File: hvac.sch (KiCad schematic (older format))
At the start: 18 parts, among them IC1 ATMEGA328P-A, J1 PROGRAMMING HEADER, J2 SERIAL PORT, U1 MIC5225

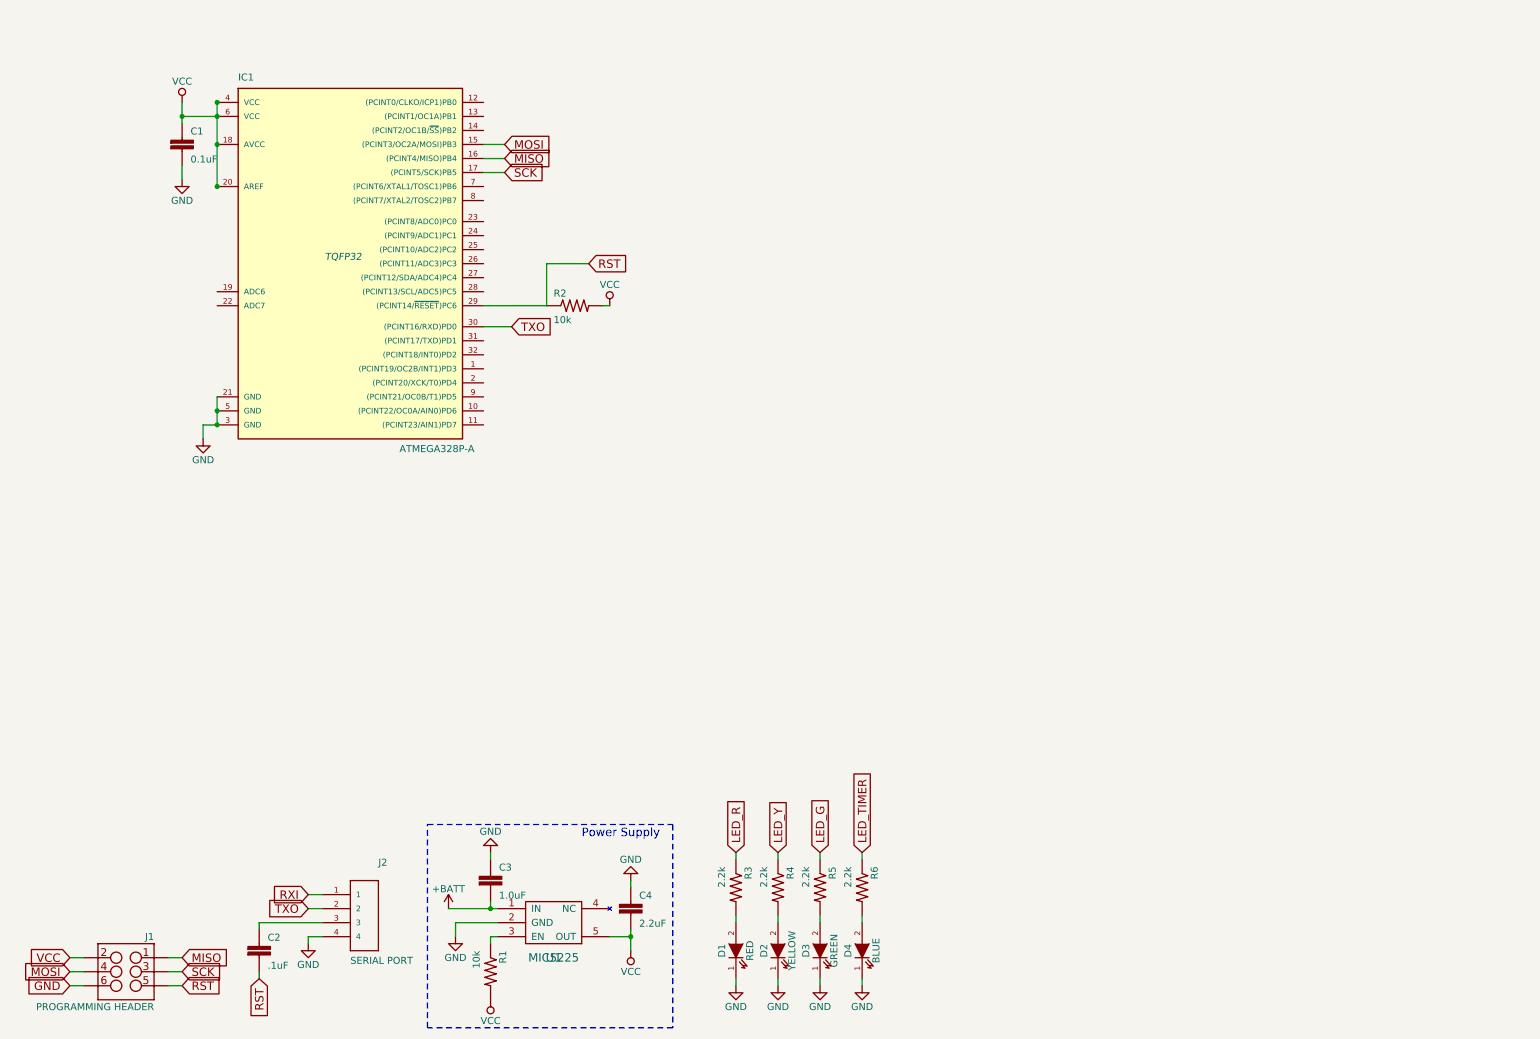
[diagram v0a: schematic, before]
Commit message: Wire up inputs and outputs
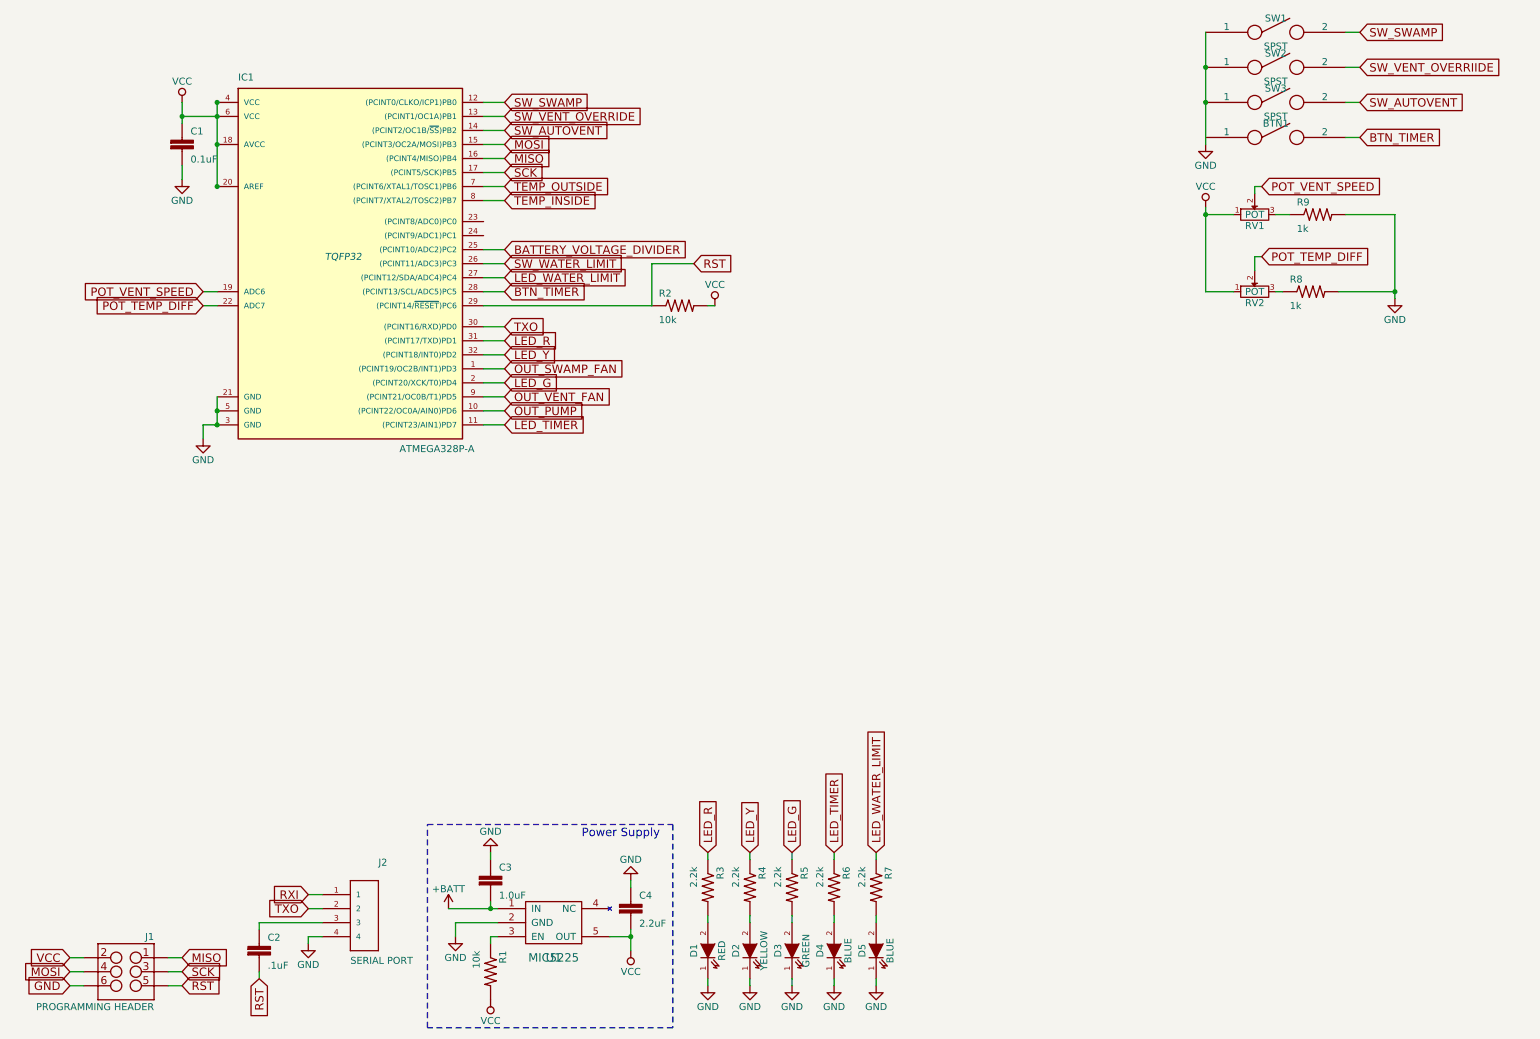
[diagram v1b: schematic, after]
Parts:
- added BTN1, SW1, SW2, SW3: SPST, symbol SPST
- added D5: BLUE, symbol LED
- added R7: 2.2k, 0402-RES, symbol RESISTOR0402
- added R8, R9: 1k, 0402-RES, symbol RESISTOR0402
- added RV1, RV2: POT, symbol POT
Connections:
- net GND: now also D5.1 (K), R8.2, R9.2, SW1.1, SW2.1, SW3.1
- net LED_G: now also IC1.2 ((PCINT20/XCK/T0)PD4)
- net LED_R: now also IC1.31 ((PCINT17/TXD)PD1)
- net LED_TIMER: now also IC1.11 ((PCINT23/AIN1)PD7)
- net LED_Y: now also IC1.32 ((PCINT18/INT0)PD2)
- net VCC: now also RV1.1, RV2.1
- net OUT_SWAMP_FAN: now reaches IC1.1 ((PCINT19/OC2B/INT1)PD3)
- net OUT_PUMP: now reaches IC1.10 ((PCINT22/OC0A/AIN0)PD6)
- net SW_SWAMP: now reaches IC1.12 ((PCINT0/CLKO/ICP1)PB0)
- net SW_SWAMP: now also SW1.2
- net SW_VENT_OVERRIDE: now reaches IC1.13 ((PCINT1/OC1A)PB1)
- net SW_AUTOVENT: now reaches IC1.14 ((PCINT2/OC1B/~SS~)PB2)
- net SW_AUTOVENT: now also SW3.2
- net POT_VENT_SPEED: now reaches IC1.19 (ADC6)
- net POT_VENT_SPEED: now also RV1.2
- net POT_TEMP_DIFF: now reaches IC1.22 (ADC7)
- net POT_TEMP_DIFF: now also RV2.2
- net BATTERY_VOLTAGE_DIVIDER: now reaches IC1.25 ((PCINT10/ADC2)PC2)
- net SW_WATER_LIMIT: now reaches IC1.26 ((PCINT11/ADC3)PC3)
- net LED_WATER_LIMIT: now reaches IC1.27 ((PCINT12/SDA/ADC4)PC4)
- net LED_WATER_LIMIT: now also R7.1
- net BTN_TIMER: now reaches IC1.28 ((PCINT13/SCL/ADC5)PC5)
- net BTN_TIMER: now also BTN1.2
- net TEMP_OUTSIDE: now reaches IC1.7 ((PCINT6/XTAL1/TOSC1)PB6)
- net TEMP_INSIDE: now reaches IC1.8 ((PCINT7/XTAL2/TOSC2)PB7)
- net OUT_VENT_FAN: now reaches IC1.9 ((PCINT21/OC0B/T1)PD5)
- new net: R9.1, RV1.3
- new net: R8.1, RV2.3
- new net: D5.2 (A), R7.2
- new net SW_VENT_OVERRIIDE: SW2.2
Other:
- moved on the sheet: D1, D2, D3, D4, R2, R3, R4, R5, R6
